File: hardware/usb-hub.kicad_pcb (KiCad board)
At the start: 4 copper layers, 49.6 x 34.5 mm, 45 parts, among them J1 USB_C_Receptacle, J2 USB_C_Receptacle, J3 USB_C_Receptacle, J4 USB_C_Receptacle, J5 USB_C_Receptacle, U1 TUSB8041, U2 TPS2561, U3 TPS2561, Y1 Crystal_GND24

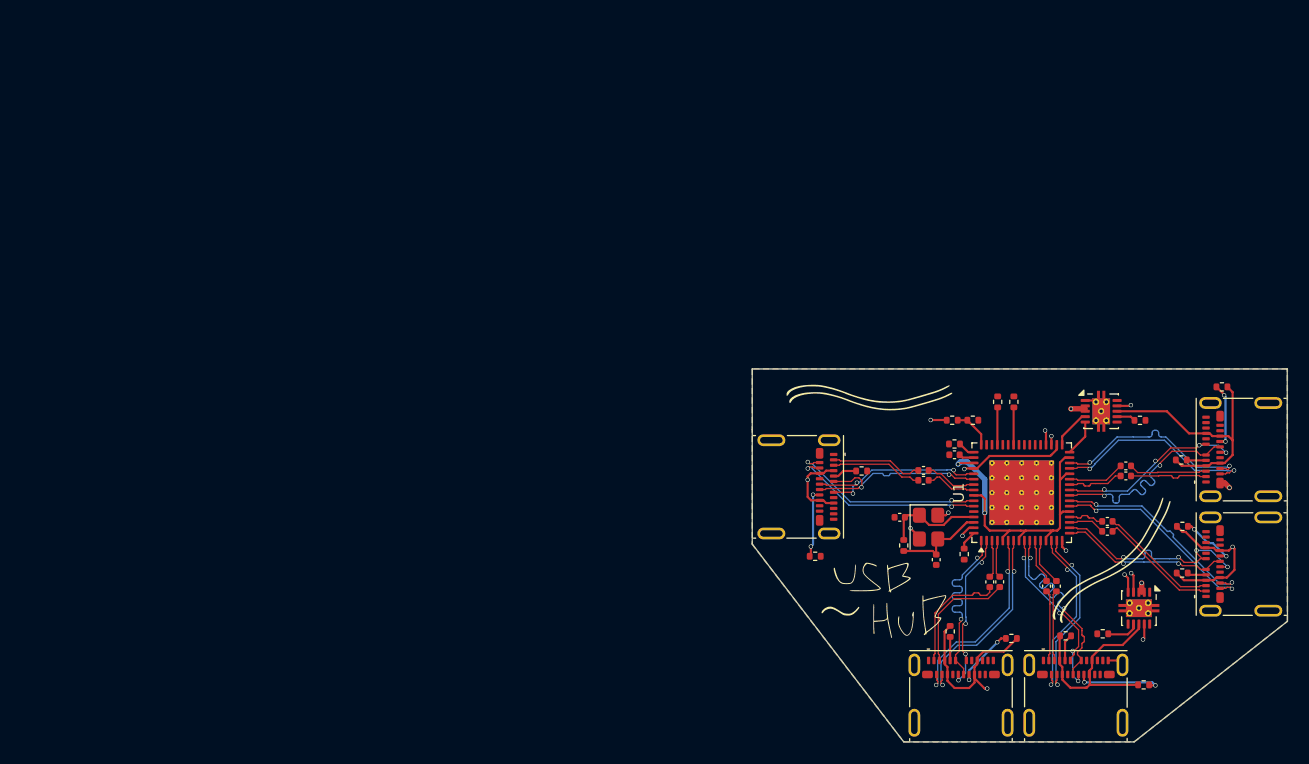
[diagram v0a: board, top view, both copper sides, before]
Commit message: PCB Changed
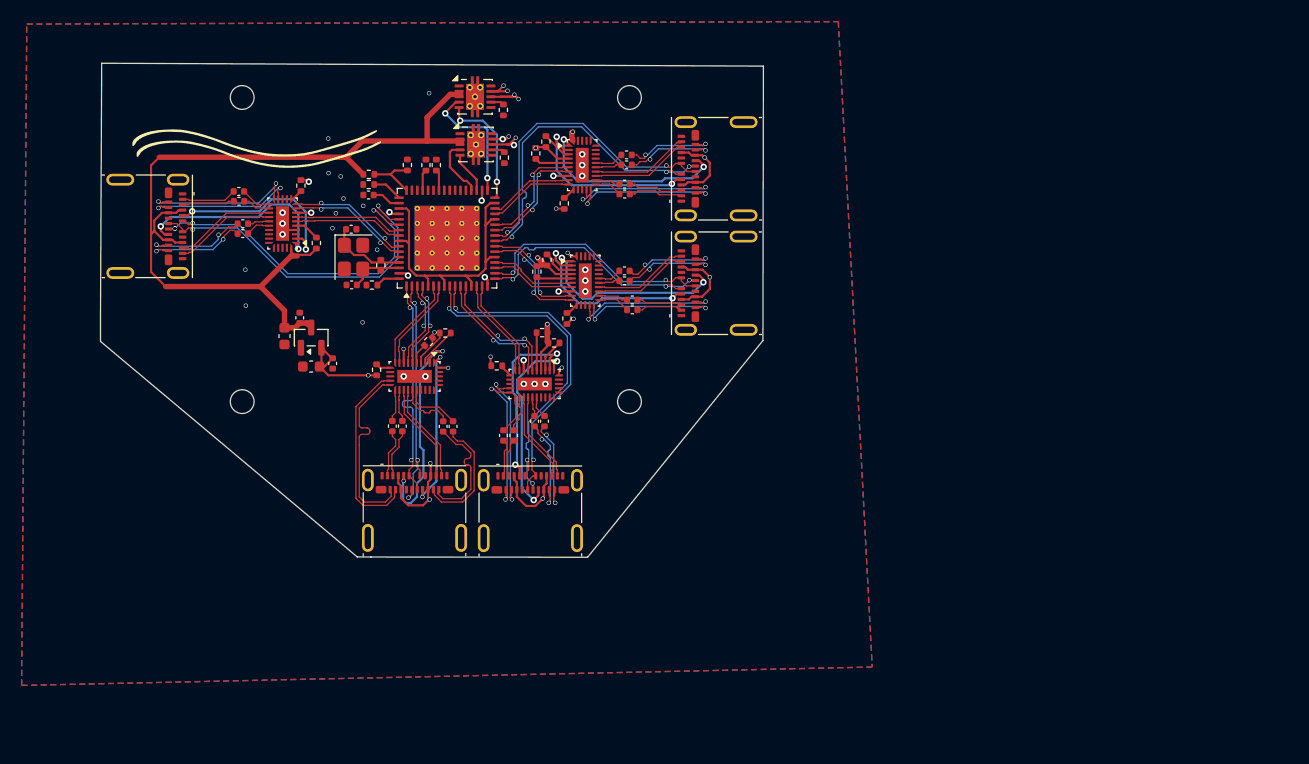
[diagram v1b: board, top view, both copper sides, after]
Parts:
- removed C10, C9: 100n, Capacitor_SMD:C_0402_1005Metric
- removed the G*** at (152.5, 100.6)
- removed the G*** at (151.1, 82.0)
- removed the G*** at (174.0, 97.1)
- removed the G*** at (170.5, 95.7)
- removed R14, R15, R16, R17, R18, R19: 5.1k, Resistor_SMD:R_0402_1005Metric
- added C14: 100n, Capacitor_SMD:C_0402_1005Metric, F.Cu at (120.0, 83.9)
- added C15: 100n, Capacitor_SMD:C_0402_1005Metric, F.Cu at (117.1, 85.2)
- added C16: 100n, Capacitor_SMD:C_0402_1005Metric, F.Cu at (120.9, 83.9)
- added C17: 100n, Capacitor_SMD:C_0402_1005Metric, F.Cu at (118.1, 85.2)
- added C18: 100n, Capacitor_SMD:C_0402_1005Metric, F.Cu at (128.3, 70.9)
- added C19: 100n, Capacitor_SMD:C_0402_1005Metric, F.Cu at (129.0, 73.6)
- added C20: 100n, Capacitor_SMD:C_0402_1005Metric, F.Cu at (128.3, 70.0)
- added C21: 100n, Capacitor_SMD:C_0402_1005Metric, F.Cu at (129.0, 72.7)
- added C22: 100n, Capacitor_SMD:C_0402_1005Metric, F.Cu at (128.5, 60.1)
- added C23: 100n, Capacitor_SMD:C_0402_1005Metric, F.Cu at (128.3, 62.8)
- added C24: 100n, Capacitor_SMD:C_0402_1005Metric, F.Cu at (128.5, 59.2)
- added C25: 100n, Capacitor_SMD:C_0402_1005Metric, F.Cu at (128.3, 61.9)
- added C26: 100n, Capacitor_SMD:C_0402_1005Metric, F.Cu at (92.6, 62.6)
- added C27: 100n, Capacitor_SMD:C_0402_1005Metric, F.Cu at (92.6, 63.5)
- added C28: 100n, Capacitor_SMD:C_0402_1005Metric, F.Cu at (93.0, 65.6)
- added C29: 100n, Capacitor_SMD:C_0402_1005Metric, F.Cu at (93.0, 66.5)
- added G***: LOGO, LOGO, F.Cu at (94.4, 59.0)
- added G***: LOGO, LOGO, B.Cu at (94.1, 73.0)
- added G***: LOGO, LOGO, B.Cu at (119.9, 70.7)
- added H1: MountingHole, MountingHole:MountingHole_2.2mm_M2, F.Cu at (128.8, 53.9)
- added H2: MountingHole, MountingHole:MountingHole_2.2mm_M2, F.Cu at (92.9, 53.9)
- added H3: MountingHole, MountingHole:MountingHole_2.2mm_M2, F.Cu at (92.9, 82.1)
- added H4: MountingHole, MountingHole:MountingHole_2.2mm_M2, F.Cu at (128.8, 82.1)
- added R20: 100k, Resistor_SMD:R_0402_1005Metric, F.Cu at (105.4, 79.1)
- added R21: 100k, Resistor_SMD:R_0402_1005Metric, F.Cu at (98.4, 62.1)
- added R22: 900k, Resistor_SMD:R_0402_1005Metric, F.Cu at (99.8, 67.4)
- added R23: 900k, Resistor_SMD:R_0402_1005Metric, F.Cu at (110.2, 76.5)
- added R24: 900k, Resistor_SMD:R_0402_1005Metric, F.Cu at (120.7, 75.7)
- added R25: 100k, Resistor_SMD:R_0402_1005Metric, F.Cu at (116.5, 78.8)
- added R26: 900k, Resistor_SMD:R_0402_1005Metric, F.Cu at (120.2, 70.0)
- added R27: 100k, Resistor_SMD:R_0402_1005Metric, F.Cu at (123.0, 74.4)
- added R28: 900k, Resistor_SMD:R_0402_1005Metric, F.Cu at (120.1, 59.1)
- added R29: 100k, Resistor_SMD:R_0402_1005Metric, F.Cu at (122.8, 63.7)
- added U4: HD3S3220, Package_DFN_QFN:Texas_RNH0030A_WQFN-30-1EP_2.5x4.5mm_P0.4mm_EP1.2x3.2mm, F.Cu at (96.7, 65.6)
- added U5: HD3S3220, Package_DFN_QFN:Texas_RNH0030A_WQFN-30-1EP_2.5x4.5mm_P0.4mm_EP1.2x3.2mm, F.Cu at (108.9, 79.7)
- added U6: MCP1700x-330xxTT, Package_TO_SOT_SMD:SOT-23, F.Cu at (99.3, 76.1)
- added U7: HD3S3220, Package_DFN_QFN:Texas_RNH0030A_WQFN-30-1EP_2.5x4.5mm_P0.4mm_EP1.2x3.2mm, F.Cu at (120.0, 80.4)
- added U8: HD3S3220, Package_DFN_QFN:Texas_RNH0030A_WQFN-30-1EP_2.5x4.5mm_P0.4mm_EP1.2x3.2mm, F.Cu at (124.7, 70.9)
- added U9: HD3S3220, Package_DFN_QFN:Texas_RNH0030A_WQFN-30-1EP_2.5x4.5mm_P0.4mm_EP1.2x3.2mm, F.Cu at (124.4, 60.2)
- C5, C8: value 100n -> 10u; footprint Capacitor_SMD:C_0402_1005Metric -> Capacitor_SMD:C_0603_1608Metric
- R10, R11, R12, R13: value 5.1k -> 10k
- moved C5 78.3 mm to (96.8, 76.0), turned to -90 degrees
- moved C6 77.1 mm to (98.2, 74.3), turned to 90 degrees
- moved C8 76.0 mm to (99.3, 78.8), turned to 180 degrees
- moved U2 74.9 mm to (114.6, 58.2), turned to 0 degrees
- moved C7 74.2 mm to (101.3, 78.5), turned to -90 degrees
- moved R8 70.8 mm to (117.2, 59.5), turned to -90 degrees
- moved R9 65.6 mm to (117.1, 55.0), turned to -90 degrees
- moved J1 64.9 mm to (84.2, 65.8)
- moved U3 64.9 mm to (114.5, 53.8)
- moved R1 60.2 mm to (104.9, 71.3), turned to 180 degrees
- moved C13 59.8 mm to (103.1, 71.3), turned to 180 degrees
- moved C11 59.4 mm to (104.6, 62.9)
- moved R2 59.3 mm to (104.6, 62.0)
- moved Y1 58.8 mm to (103.2, 68.7)
- moved R13 58.8 mm to (121.1, 58.0), turned to 90 degrees
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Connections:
- net /USBUP_DN renamed /USBUFP_DN
- net /USBUP_DP renamed /USBUFP_DP
- C1 pad 1: /TX_1P -> /DFP1TX1N
- C1 pad 2: /SSTX1P -> /1TX1N
- C2 pad 1: /TX_1N -> /DFP1TX1P
- C2 pad 2: /SSTX1N -> /1TX1P
- C3 pad 1: /TX_2P -> /DFP1TX2N
- C3 pad 2: /SSTX2P -> /1TX2P
- C4 pad 1: /TX_2N -> /DFP1TX2P
- C4 pad 2: /SSTX2N -> /1TX2N
- C5 pad 1: /TX_3P -> VBUS
- C5 pad 2: /SSTX3P -> GND
- C6 pad 1: /TX_3N -> VBUS
- C6 pad 2: /SSTX3N -> GND
- C7 pad 1: /TX_4P -> +3V3
- C7 pad 2: /SSTX4P -> GND
- C8 pad 1: /TX_4N -> +3V3
- C8 pad 2: /SSTX4N -> GND
- J1 pad A10: unconnected-(J1-RX2--PadA10) -> /UFPRX2N
- J1 pad A11: unconnected-(J1-RX2+-PadA11) -> /UFPRX2P
- J1 pad A2: /SSTXUPP -> /0UFPTX1N
- J1 pad A3: /SSTXUPN -> /0UFPTX1P
- J1 pad B10: /SSRXUPN -> /UFPRX1N
- J1 pad B11: /SSRXUPP -> /UFPRX1P
- J1 pad B2: unconnected-(J1-TX2+-PadB2) -> /0UFPTX2P
- J1 pad B3: unconnected-(J1-TX2--PadB3) -> /0UFPTX2N
- J2 pad A10: unconnected-(J2-RX2--PadA10) -> /DFP1RX2N
- J2 pad A11: unconnected-(J2-RX2+-PadA11) -> /DFP1RX2P
- J2 pad A2: /SSTX1P -> /1TX1N
- J2 pad A3: /SSTX1N -> /1TX1P
- J2 pad B10: /SSRX1N -> /DFP1RX1N
- J2 pad B11: /SSRX1P -> /DFP1RX1P
- J2 pad B2: unconnected-(J2-TX2+-PadB2) -> /1TX2P
- J2 pad B3: unconnected-(J2-TX2--PadB3) -> /1TX2N
- J3 pad A10: unconnected-(J3-RX2--PadA10) -> /DFP2RX2N
- J3 pad A11: unconnected-(J3-RX2+-PadA11) -> /DFP2RX2P
- J3 pad A2: /SSTX2P -> /2TX1N
- J3 pad A3: /SSTX2N -> /2TX1P
- J3 pad B10: /SSRX2N -> /DFP2RX1N
- J3 pad B11: /SSRX2P -> /DFP2RX1P
- J3 pad B2: unconnected-(J3-TX2+-PadB2) -> /2TX2P
- J3 pad B3: unconnected-(J3-TX2--PadB3) -> /2TX2N
- J4 pad A10: unconnected-(J4-RX2--PadA10) -> /DFP3RX2N
- J4 pad A11: unconnected-(J4-RX2+-PadA11) -> /DFP3RX2P
- J4 pad A2: /SSTX3P -> /3TX1N
- J4 pad A3: /SSTX3N -> /3TX1P
- J4 pad B10: /SSRX3N -> /DFP3RX1N
- J4 pad B11: /SSRX3P -> /DFP3RX1P
- J4 pad B2: unconnected-(J4-TX2+-PadB2) -> /3TX2P
- J4 pad B3: unconnected-(J4-TX2--PadB3) -> /3TX2N
- J5 pad A10: unconnected-(J5-RX2--PadA10) -> /DFP4RX2N
- J5 pad A11: unconnected-(J5-RX2+-PadA11) -> /DFP4RX2P
- J5 pad A2: /SSTX4P -> /4TX1N
- J5 pad A3: /SSTX4N -> /4TX1P
- J5 pad B10: /SSRX4N -> /DFP4RX1N
- J5 pad B11: /SSRX4P -> /DFP4RX1P
- J5 pad B2: unconnected-(J5-TX2+-PadB2) -> /4TX2P
- J5 pad B3: unconnected-(J5-TX2--PadB3) -> /4TX2N
- R10 pad 1: Net-(J1-CC2) -> /VBUS_1
- R10 pad 2: GND -> Net-(U5-CURRENT_MODE)
- R11 pad 1: Net-(J1-CC1) -> /VBUS_2
- R11 pad 2: GND -> Net-(U7-CURRENT_MODE)
- R12 pad 1: /VBUS_1 -> /VBUS_3
- R12 pad 2: Net-(J2-CC2) -> Net-(U8-CURRENT_MODE)
- R13 pad 1: /VBUS_1 -> /VBUS_4
- R13 pad 2: Net-(J2-CC1) -> Net-(U9-CURRENT_MODE)
- U1 pad 11: /TX_2P -> /SSTX2P
- U1 pad 12: /TX_2N -> /SSTX2N
- U1 pad 19: /TX_3P -> /SSTX3P
- U1 pad 20: /TX_3N -> /SSTX3N
- U1 pad 26: /TX_4P -> /SSTX4P
- U1 pad 27: /TX_4N -> /SSTX4N
- U1 pad 3: /TX_1P -> /SSTX1P
- U1 pad 4: /TX_1N -> /SSTX1N
- U1 pad 55: /TX_0P -> /SSTXUFPP
- U1 pad 56: /TX_0N -> /SSTXUFPN
- U1 pad 58: /SSRXUPP -> /SSRXUFPP
- U1 pad 59: /SSRXUPN -> /SSRXUFPN
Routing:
- net +3V3: track 28.7 -> 103.2 mm, vias 3 -> 14
- net /VBUS_2: track 20.2 -> 56.3 mm, vias 0 -> 5
- net /VBUS_1: track 37.3 -> 59.3 mm, vias 2 -> 6
- net /VBUS_3: track 38.3 -> 57.9 mm, vias 2 -> 5
- net Net-(J2-CC1): track 2.18 -> 20.9 mm, vias 0 -> 2
- net /SSRXUPP: track 18.3 -> 0.00 mm, vias 2 -> 0
- net /SSRXUPN: track 18.3 -> 0.00 mm, vias 2 -> 0
- net /DFP1RX1N: track 0.00 -> 17.6 mm
- net /DFP1RX1P: track 0.00 -> 17.5 mm
- net VBUS: track 64.7 -> 81.4 mm, vias 4 -> 0
- net Net-(J4-CC1): track 1.77 -> 17.7 mm, vias 0 -> 2
- net Net-(J5-CC1): track 1.79 -> 17.3 mm, vias 0 -> 2
- net Net-(J1-CC1): track 2.27 -> 17.7 mm, vias 0 -> 2
- net /CTRL_1: track 20.7 -> 5.58 mm, vias 2 -> 0
- net Net-(J3-CC1): track 2.51 -> 17.4 mm, vias 0 -> 2
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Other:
- board size 49.6 x 34.5 mm -> 61.4 x 45.8 mm
- board text removed: "Exit 1"
- board text removed: "Exit 2"
- board text removed: "Exit 3"
- board text removed: "Exit 4"
- board text removed: "SUUUUPER SPEED"
- board text removed: "bits, enter here"
